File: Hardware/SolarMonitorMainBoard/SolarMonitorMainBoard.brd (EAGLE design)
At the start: 100 x 80 mm, 28 parts, among them K1 RT314F12, U1 INA219AIDR, U2 INA219AIDR, U3 INA219AIDR, U4 INA219AIDR, U5 INA219AIDR, U6 TSR_1-2450, X1 MKDS_5/3-7,62, X2 MKDS_5/3-7,62, X3 MKDS_5/3-7,62, X4 MKDS_5/3-7,62

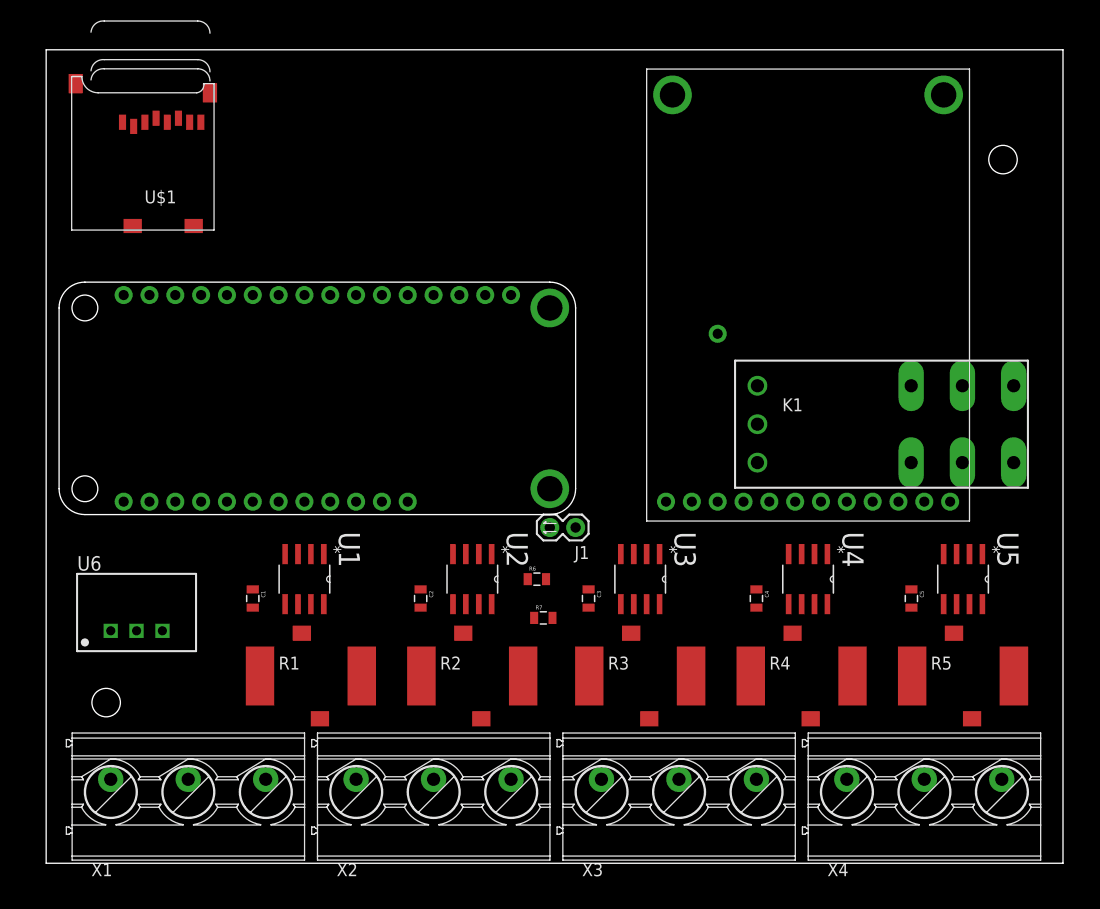
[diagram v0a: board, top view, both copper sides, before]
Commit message: Work in progress on the main board ...
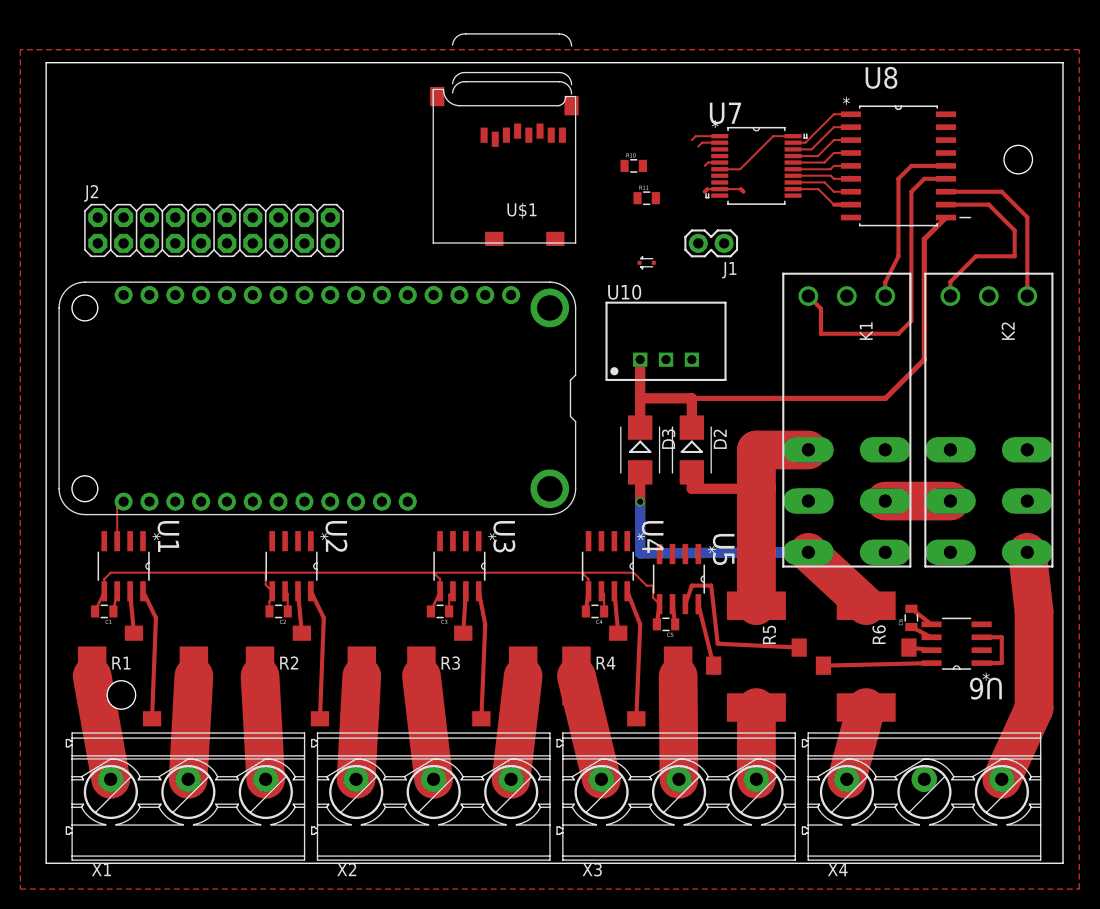
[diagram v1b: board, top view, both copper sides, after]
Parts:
- removed MS2: FONA, BtParts:FONA
- removed R7: (no value), SparkFun-Resistors:0805
- added C6: (no value), SparkFun-Capacitors:0805
- added D2, D3: (no value), diode:SMB
- added J2: (no value), SparkFun-Connectors:2X10
- added K2: RT314F12, relay:RT1-BI
- added R10, R11: (no value), SparkFun-Resistors:0805
- added U10: TSR_1-2450, _traco_tsr-1:TSR-1
- added U7: MCP23008-E/SS, Microchip_By_element14_Batch_1:SOP65P780X200-20N
- added U8: ULN2803ADW, Texas Instruments_By_element14_Batch_1:SOIC127P1030X265-18N
- MS1: value FEATHERWING -> FEATHERWING_NODIM; device adafruit:FEATHERWING -> adafruit:FEATHERWING_DIM
- R6: value (none) -> 5m; device SparkFun-Resistors:0805 -> resistor-shunt:SMV
- U6: value TSR_1-2450 -> INA219AIDR; device _traco_tsr-1:TSR-1 -> Texas Instruments_By_element14_Batch_1:SOIC127P600X175-8N
- moved U6 80.7 mm to (89.5, 21.6), turned to 180 degrees
- moved U$1 35.6 mm to (52.1, 61.0)
- moved R6 33.3 mm to (80.6, 20.3), turned to 270 degrees
- moved J1 31.5 mm to (66.7, 61.0)
- moved U5 27.9 mm to (62.2, 27.9)
- moved D1 27.7 mm to (59.1, 59.1)
- moved C5 24.3 mm to (61.0, 23.5), turned to 180 degrees
- moved R5 20.4 mm to (69.8, 20.3), turned to 270 degrees
- moved U4 19.7 mm to (55.2, 29.2)
- moved U3 17.8 mm to (40.6, 29.2)
- moved U1 17.8 mm to (7.62, 29.2)
- moved U2 17.8 mm to (24.1, 29.2)
- moved R4 17.1 mm to (57.1, 18.4)
- moved R3 16.5 mm to (41.9, 18.4)
- moved R1 16.5 mm to (9.53, 18.4)
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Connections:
- new net FONA_RX: J2.8, MS1.15
- new net FONA_TX: J2.6, MS1.14
- new net LIN1: D2.A, K1.12B, R5.I2
- new net LIN2: D3.A, K1.14B, R6.I2
- new net LOUT: K2.14A, X4.3
- new net N$21: R6.I1, X4.1
- new net N$22: K1.11A, K2.11B
- new net N$23: R6.U1, U6.8
- new net N$24: R6.U2, U6.7
- new net N$25: U7.16, U8.4
- new net N$26: U7.15, U8.5
- new net N$27: U7.14, U8.6
- new net N$28: U7.13, U8.7
- new net N$29: U7.12, U8.8
- new net N$30: K2.A1, U8.11
- new net N$31: K2.A2, U8.12
- new net N$32: K1.A1, U8.13
- new net N$33: K1.A2, U8.14
- net 1VIN+: now also X1.2; no longer X2.1
- net 1VIN-: now also X1.1; no longer X1.3
- net 5V: now also J2.2, U10.3; no longer MS2.99, U6.3
- net FONA_BAT: now also J2.4; no longer MS2.1
- net FONA_RST: now also J2.10; no longer MS2.5
- net GND: now also C6.1, J2.1, K1.A3, K2.A3, U10.2, U6.6, U7.3, U7.4, U7.5, U7.9, U8.9; no longer MS2.2, X1.2
- net N$1: now also X1.3; no longer X2.2
- net N$10: now also U7.17, U8.3; no longer R5.I2, X4.2
- net N$2: now also U7.19, U8.1; no longer MS1.15, MS2.10
- net N$3: now also U7.18, U8.2; no longer MS1.14, MS2.9
- net N$4: now also X2.1; no longer X2.3
- net N$5: now also X2.3; no longer X3.2
- net N$6: now also X2.2; no longer X3.1
- net N$7: now also X3.1; no longer X3.3
- net N$8: now also X3.2; no longer X4.1
- net N$9: now also X3.3; no longer X4.3
- net SCL: now also R10.1, U6.4, U7.1; no longer R6.1
- net SDA: now also R11.2, U6.1, U6.3, U7.2; no longer R7.2
- net VCC: now also C6.2, J2.3, R10.2, R11.1, U6.5, U7.20, U7.6; no longer MS2.12, R6.2, R7.1
- net VI: now also D2.C, D3.C, U10.1, U8.10; no longer U6.1, X1.1
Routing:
- net VCC: track 0.00 -> 85.8 mm
- net VI: track 0.00 -> 53.9 mm
- net LIN2: track 0.00 -> 32.2 mm, vias 0 -> 1
- net N$32: track 0.00 -> 30.3 mm
- net LIN1: track 0.00 -> 28.4 mm
- net LOUT: track 0.00 -> 23.1 mm
- net N$30: track 0.00 -> 19.1 mm
- net GND: track 0.00 -> 18.2 mm
- net N$20: track 0.00 -> 17.6 mm
- net N$33: track 0.00 -> 17.0 mm
- net N$31: track 0.00 -> 16.8 mm
- net SDA: track 0.00 -> 12.9 mm
- net N$13: track 0.00 -> 12.8 mm
- net N$11: track 0.00 -> 12.8 mm
- net N$17: track 0.00 -> 12.8 mm
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- added copper zone on layer 1, net GND
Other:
- board size 100 x 80 mm -> 100 x 78.7 mm
